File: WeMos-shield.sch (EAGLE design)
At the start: 23 parts, among them Q1 N-MOS

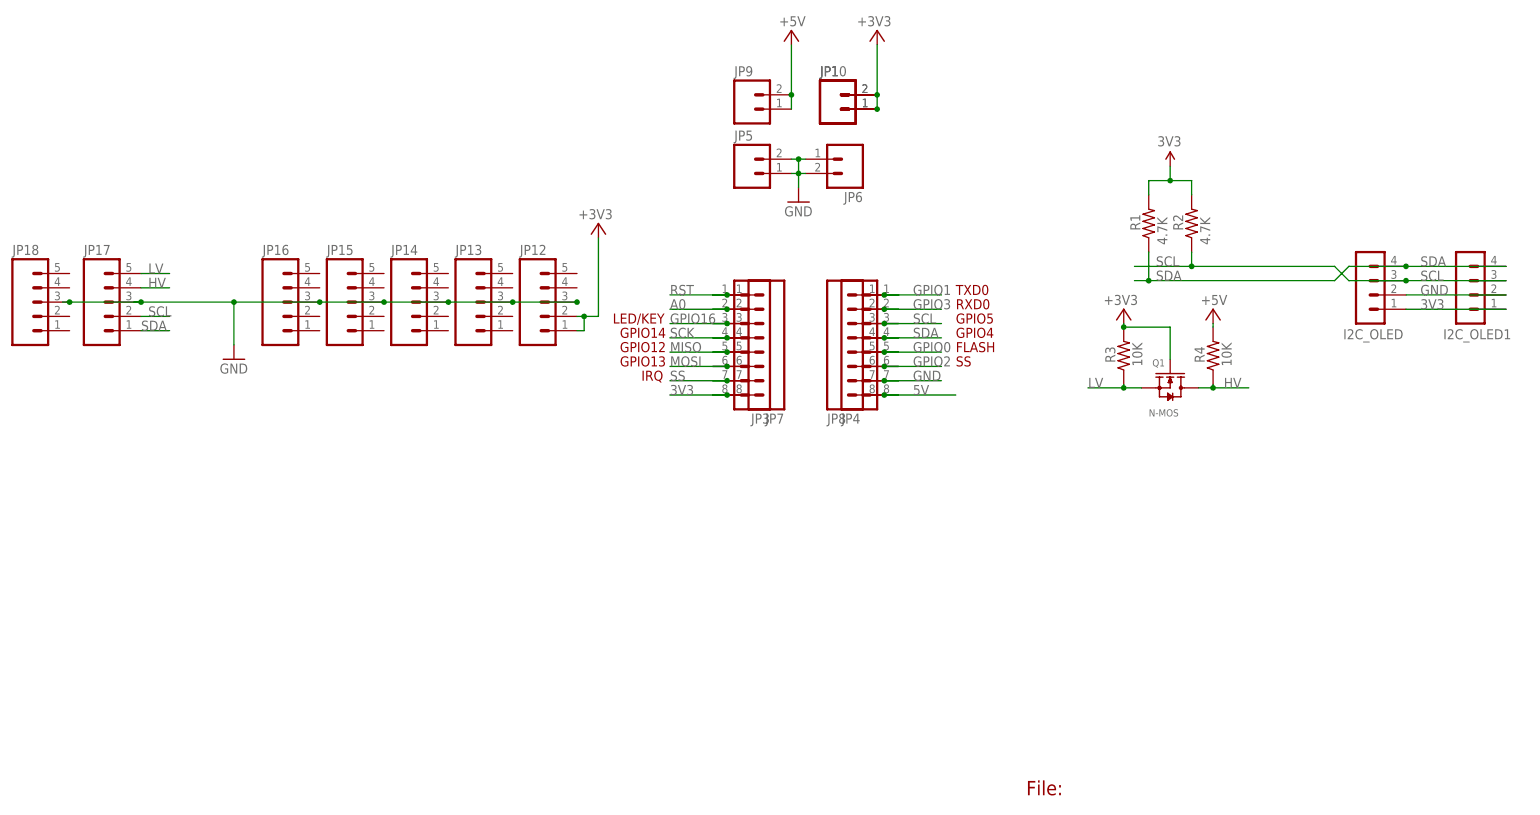
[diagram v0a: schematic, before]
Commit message: Version 1.1
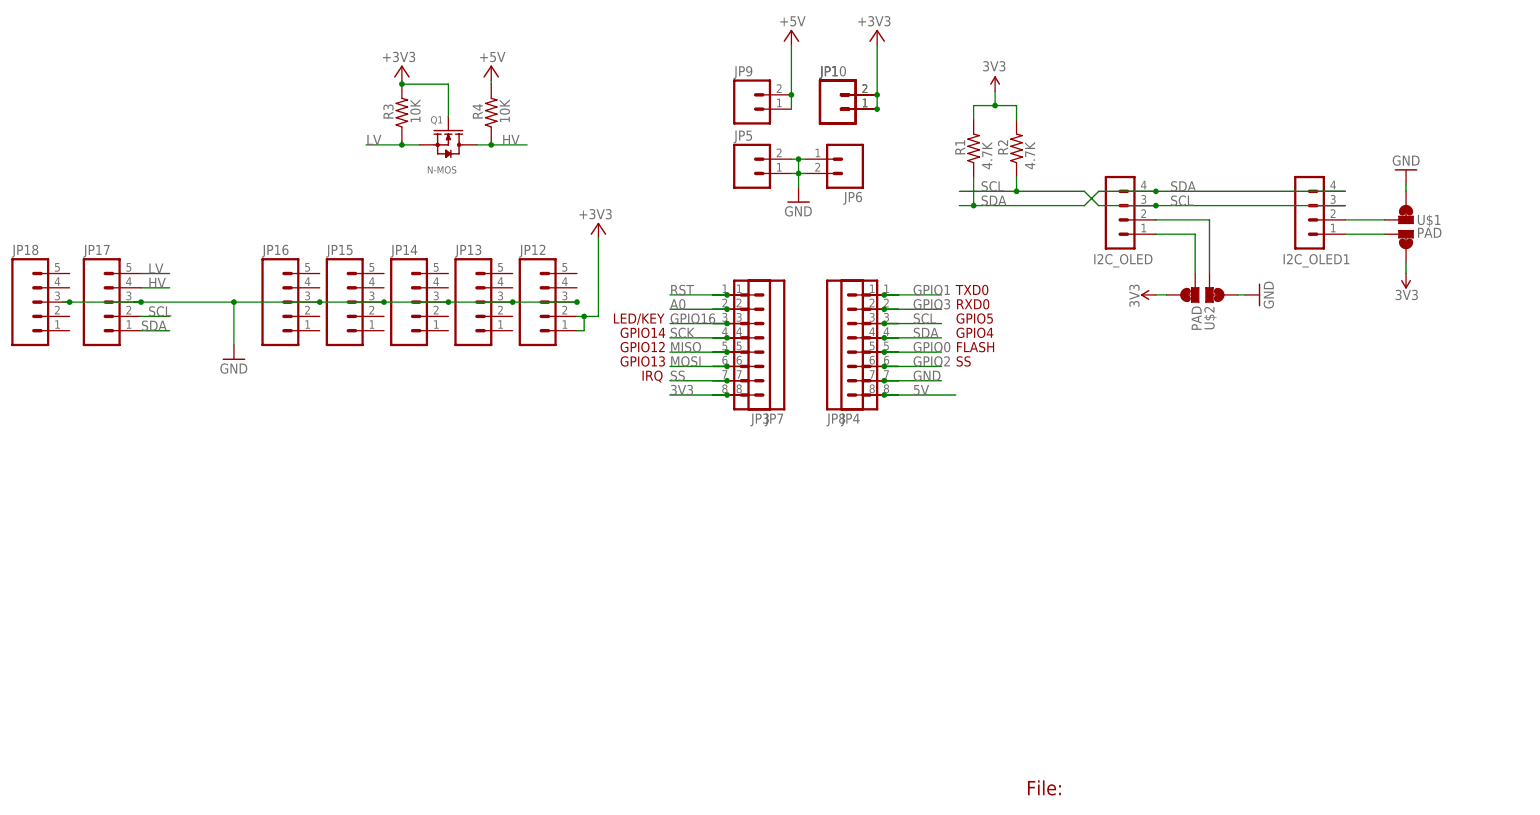
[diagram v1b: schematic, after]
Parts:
- added U$1, U$2: PAD, _c2h:PAD-JUMPER-SWAPSWAP
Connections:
- new net V+J: I2C_OLED.1, U$2.3
- new net V+O: I2C_OLED1.1, U$1.3
- new net V-J: I2C_OLED.2, U$2.2
- new net V-O: I2C_OLED1.2, U$1.2
- net 3V3: now also U$1.4, U$2.4; no longer I2C_OLED.1, I2C_OLED1.1
- net GND: now also U$1.1, U$2.1; no longer I2C_OLED.2, I2C_OLED1.2
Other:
- moved on the sheet: I2C_OLED, I2C_OLED1, Q1, R1, R2, R3, R4
